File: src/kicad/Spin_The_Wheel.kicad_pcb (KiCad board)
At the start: 2 copper layers, 100 x 100 mm, 42 parts, among them J1 USB_A, Q1 NPN, Q2 NPN, Q3 NPN, Q5 PNP, Q6 PNP, SW1 START, SW2 STOP, U1 ICM7555xB, U2 4017

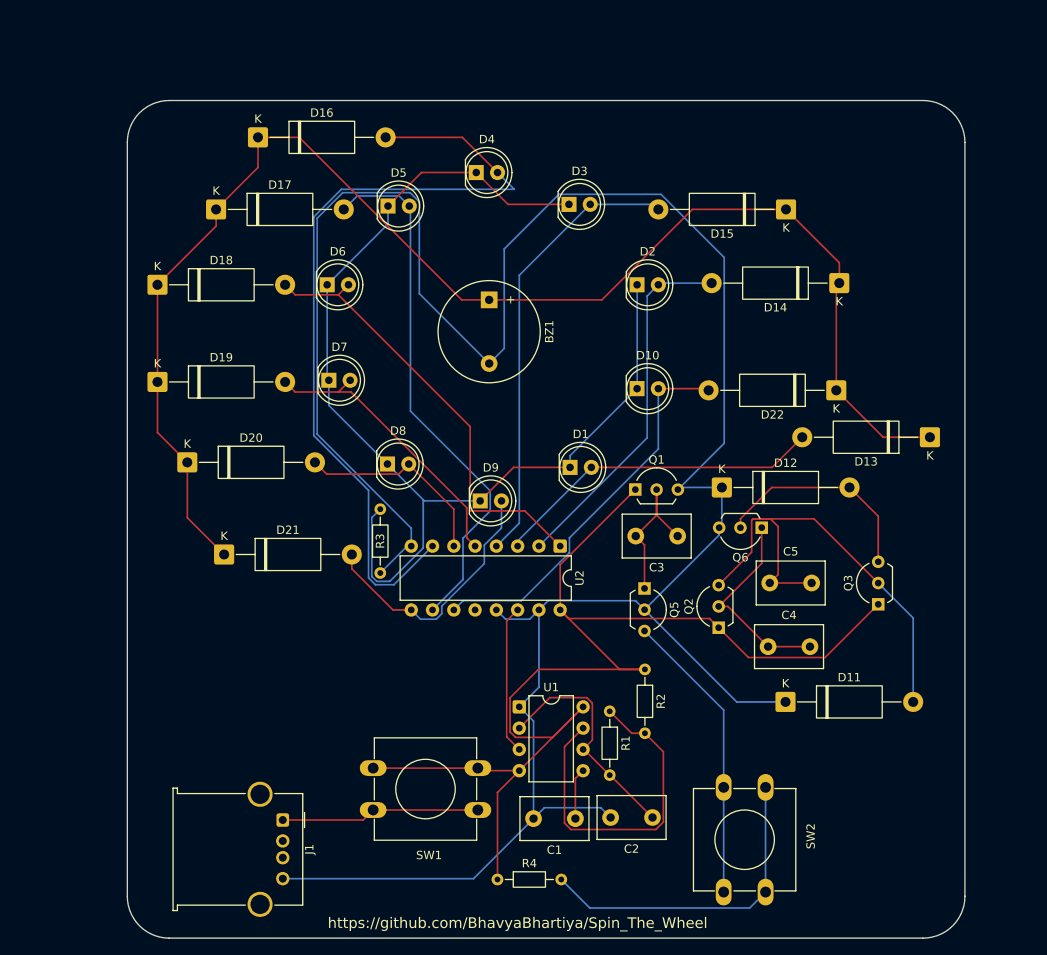
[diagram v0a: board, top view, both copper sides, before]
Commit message: Add files via upload
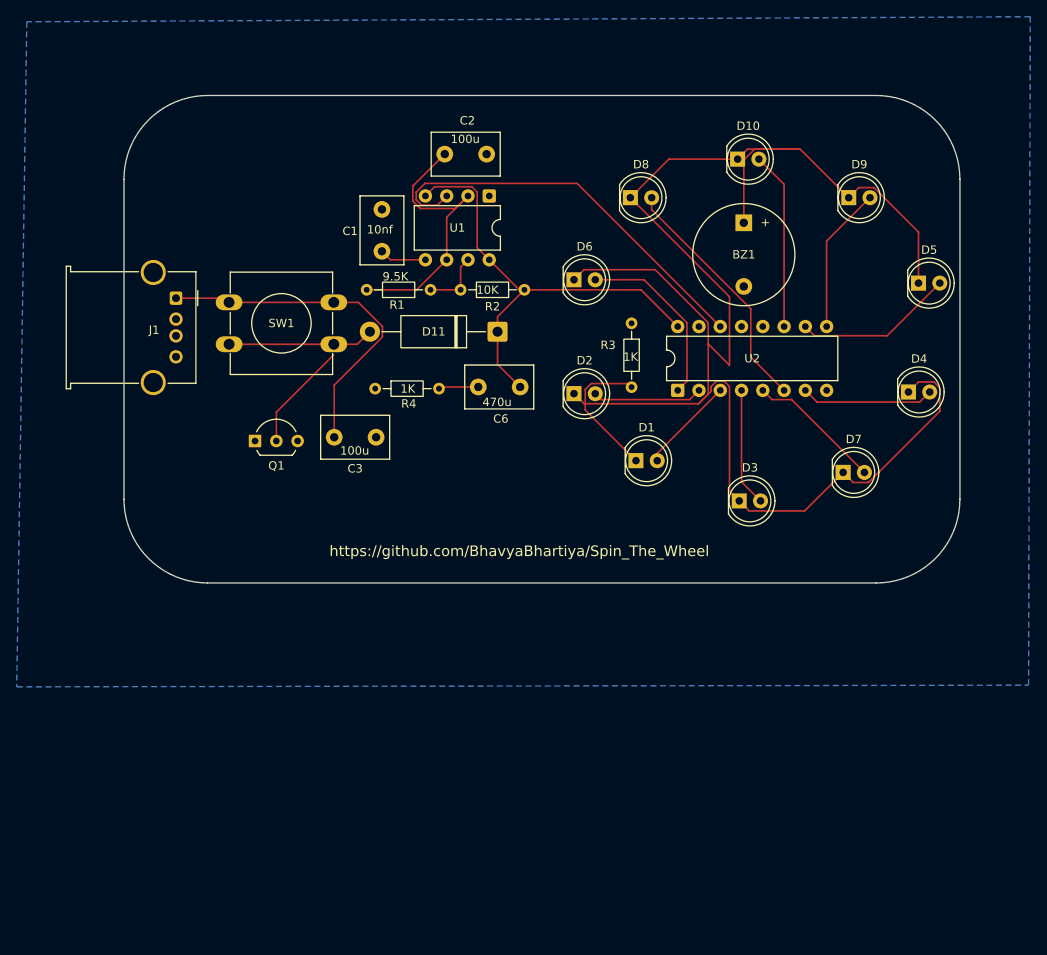
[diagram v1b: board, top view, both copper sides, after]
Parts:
- removed C4: 68uf, Capacitor_THT:C_Disc_D8.0mm_W5.0mm_P5.00mm
- removed C5: 100uf, Capacitor_THT:C_Disc_D8.0mm_W5.0mm_P5.00mm
- removed D12, D13, D14, D15, D16, D17, D18, D19, D20, D21, D22: D, Diode_THT:D_DO-15_P15.24mm_Horizontal
- removed Q2, Q3: NPN, Package_TO_SOT_THT:TO-92L_Inline_Wide
- removed Q5, Q6: PNP, Package_TO_SOT_THT:TO-92L_Inline_Wide
- removed SW2: STOP, Button_Switch_THT:SW_PUSH-12mm
- added C6: 470uf, Capacitor_THT:C_Disc_D8.0mm_W5.0mm_P5.00mm, F.Cu at (119.3, 84.6)
- C3: value 33uf -> 100uf
- Q1: value NPN -> Q_PNP
- R4: value 10K -> 1K
- SW1: value START -> START/STOP
- moved C2 83.0 mm to (110.3, 56.8), turned to 0 degrees
- moved C1 71.6 mm to (102.8, 68.4), turned to 90 degrees
- moved SW1 67.5 mm to (84.5, 74.5), turned to 0 degrees
- moved D5 64.0 mm to (166.9, 72.2)
- moved J1 63.6 mm to (78.2, 74.0)
- moved D7 62.4 mm to (157.9, 94.8)
- moved U1 61.1 mm to (115.6, 61.8), turned to -90 degrees
- moved R4 60.4 mm to (102.0, 84.8)
- moved D4 57.9 mm to (165.7, 85.2)
- moved D9 57.0 mm to (158.5, 62.0)
- moved D11 56.0 mm to (116.6, 78.0), turned to 180 degrees
- moved R1 54.7 mm to (108.6, 73.0), turned to 180 degrees
- moved R2 47.5 mm to (119.8, 73.0), turned to 180 degrees
- moved Q1 45.8 mm to (87.7, 91.0)
- moved D8 43.0 mm to (132.5, 62.0)
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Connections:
- C3 pad 1: Net-(Q1-B) -> GND
- C3 pad 2: Net-(Q1-B) -> Net-(J1-VBUS)
- D1 pad 1: Net-(D1-K) -> Net-(BZ1-+)
- D10 pad 1: Net-(D1-K) -> Net-(BZ1-+)
- D11 pad 1: GND -> VCC
- D2 pad 1: Net-(D1-K) -> Net-(BZ1-+)
- D3 pad 1: Net-(D1-K) -> Net-(BZ1-+)
- D4 pad 1: Net-(D1-K) -> Net-(BZ1-+)
- D5 pad 1: Net-(D1-K) -> Net-(BZ1-+)
- D6 pad 1: Net-(D1-K) -> Net-(BZ1-+)
- D7 pad 1: Net-(D1-K) -> Net-(BZ1-+)
- D8 pad 1: Net-(D1-K) -> Net-(BZ1-+)
- D9 pad 1: Net-(D1-K) -> Net-(BZ1-+)
- Q1 pad 1: VCC -> (no net)
- Q1 pad 2: Net-(Q1-B) -> (no net)
- Q1 pad 3: GND -> (no net)
- R3 pad 2: Net-(D1-K) -> Net-(BZ1-+)
- R4 pad 1: VCC -> GND
- SW1 pad 2: VCC -> Net-(D11-A)
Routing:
- net GND: track 296.4 -> 0.00 mm
- net Net-(D1-K): track 134.2 -> 0.00 mm
- net VCC: track 148.6 -> 55.4 mm
- net Net-(D4-A): track 98.9 -> 15.9 mm
- net Net-(D5-A): track 64.1 -> 19.1 mm
- net Net-(D11-A): track 59.2 -> 17.4 mm
- net Net-(D3-A): track 53.8 -> 14.1 mm
- net Net-(BZ1-+): track 171.5 -> 210.2 mm
- net Net-(Q5-E): track 35.1 -> 0.00 mm
- net Net-(C6-Pad2): track 39.1 -> 4.77 mm
- net Net-(U1-DISCH): track 41.5 -> 7.54 mm
- net Net-(D6-A): track 53.4 -> 21.6 mm
- net Net-(U1-OUT): track 17.8 -> 49.1 mm
- net Net-(D2-A): track 43.5 -> 13.1 mm
- net Net-(D1-A): track 39.7 -> 11.5 mm
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- added copper zone on B.Cu, net GND
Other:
- board size 100 x 100 mm -> 99.8 x 58.2 mm
- board text added: "100u"
- board text added: "10K"
- board text added: "10nf"
- board text added: "1K"
- board text added: "470u"
- board text added: "9.5K"
